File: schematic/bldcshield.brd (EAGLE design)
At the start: 51 parts, among them IC3 IR2101SMD, IC4 IR2101SMD, IC5 IR2101SMD

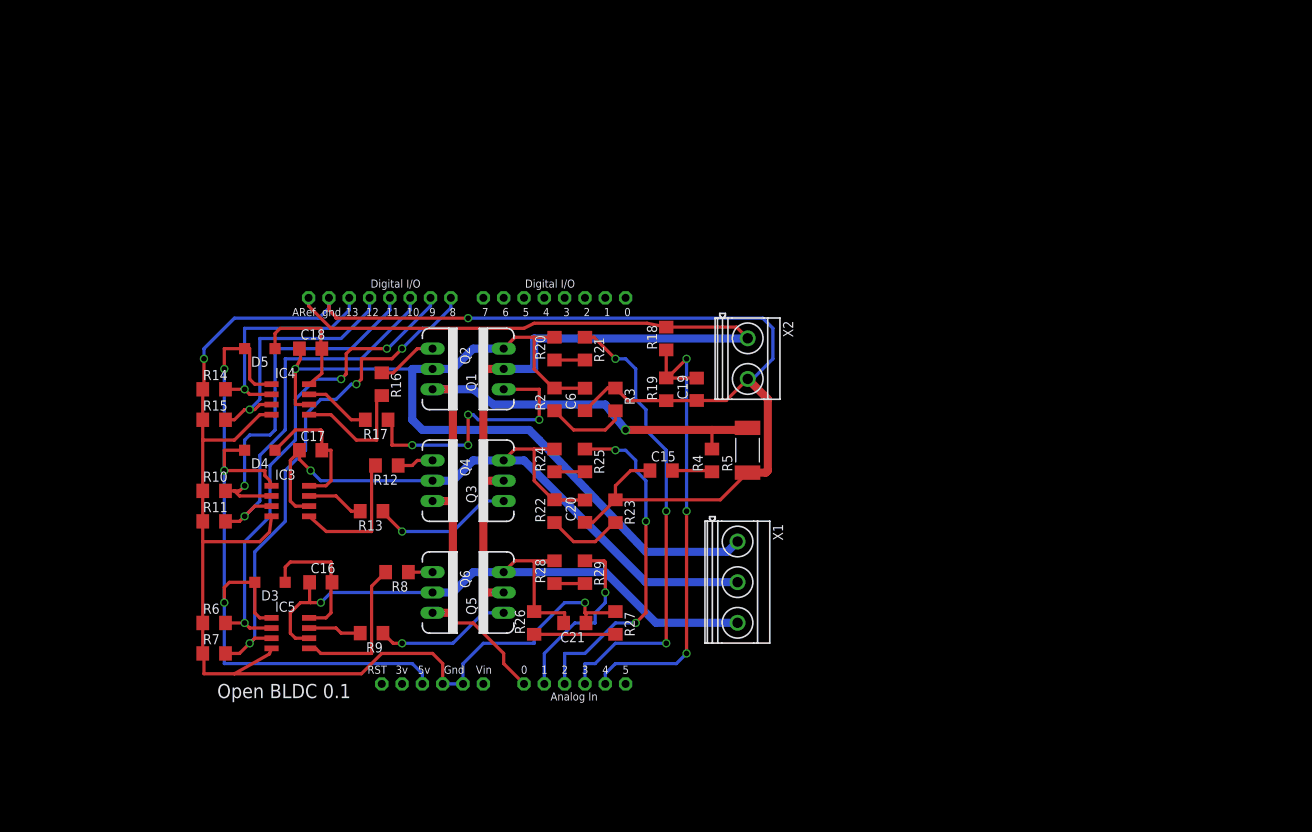
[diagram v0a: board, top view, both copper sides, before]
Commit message: redoing brf layout from scatch
deleted gerbers and backed up brd file
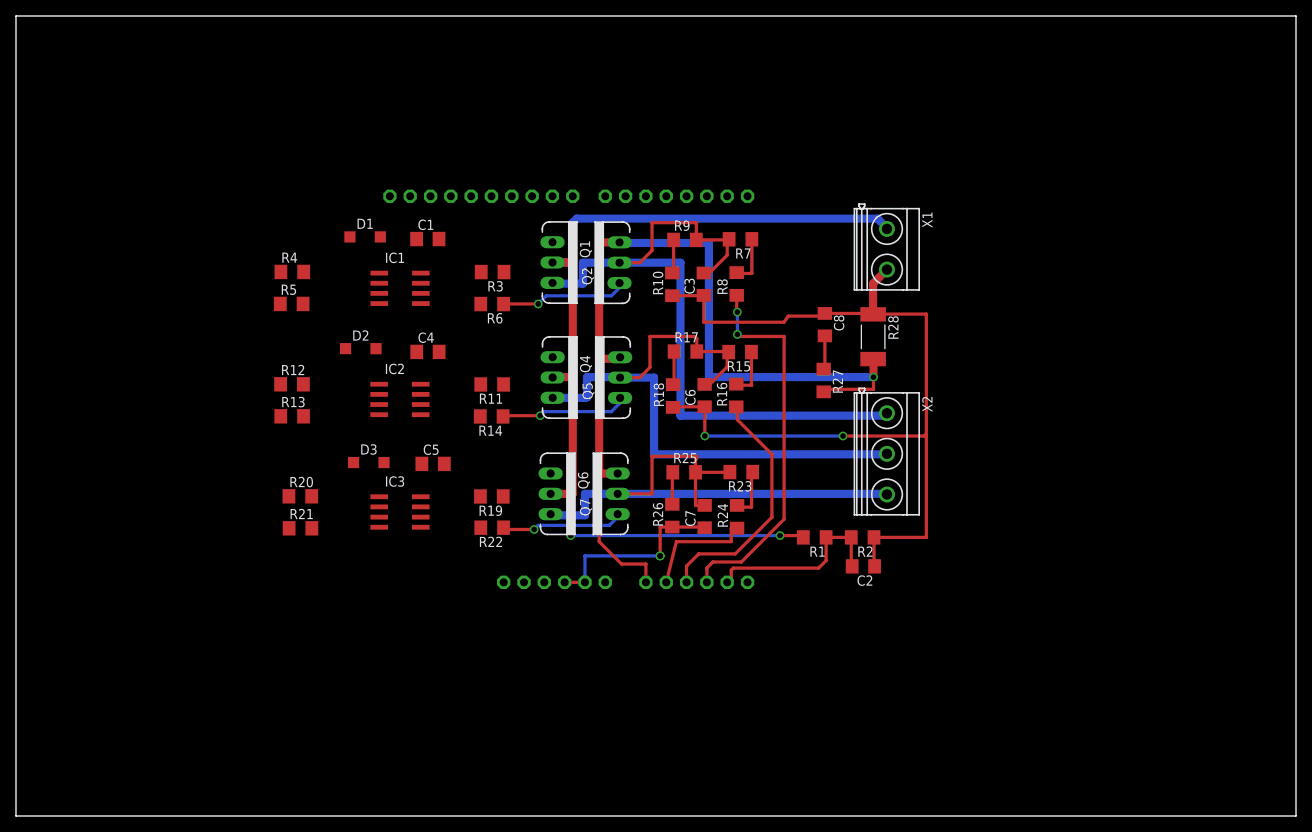
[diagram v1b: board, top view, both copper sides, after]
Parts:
- removed C15, C19: 22p, SmartPrj:C1206
- removed C16, C17, C18: 100nf, SmartPrj:C1206
- removed C20, C21: 100pF, SmartPrj:C1206
- removed D4, D5: MMSD914, diode:SOD123
- removed E$1: (no value), adafruit:ARDUINO-NOHOLE
- removed IC4, IC5: IR2101SMD, IR:SO08
- removed R29: 15k, SmartPrj:R1206
- added C1, C4, C5: 100nf, SmartPrj:C1206
- added C2, C8: 22p, SmartPrj:C1206
- added C3, C7: 100pF, SmartPrj:C1206
- added D1, D2: MMSD914, diode:SOD123
- added IC1, IC2: IR2101SMD, IR:SO08
- added Q7: (no value), SparkFun:TO220V
- added R1: 200K, SmartPrj:R1206
- Q3: value (none) -> Shield; device SparkFun:TO220V -> adafruit:ARDUINOR3-BLDC
- R10: value 10k -> 22k
- R11, R14, R6: value 10k -> 22
- R12, R13: value 22 -> 10k
- R15, R7: value 10k -> 100k
- R16, R8: value 22 -> 15k
- R17, R9: value 22 -> 22k
- R18: value 200K -> 22k
- R19: value 68k -> 22
- R2: value 22k -> 68k
- R20: value 100k -> 10k
- R21: value 15k -> 10k
- R22, R3: value 22k -> 22
- R23: value 22k -> 100k
- R24: value 100k -> 15k
- R25: value 15k -> 22k
- R27: value 22k -> 4.7k
- R28: value 100k -> 0.001; device SmartPrj:R1206 -> resistor:R2512
- R4: value 4.7k -> 10k
- R5: value 0.001 -> 10k; device resistor:R2512 -> SmartPrj:R1206
- X1: device con-phoenix-508:MKDSN1,5/3-5,08 -> con-phoenix-508:MKDSN1,5/2-5,08
- X2: device con-phoenix-508:MKDSN1,5/2-5,08 -> con-phoenix-508:MKDSN1,5/3-5,08
- moved R7 83.7 mm to (90.6, 72.1), turned to 180 degrees
- moved R15 66.3 mm to (90.5, 58.0), turned to 180 degrees
- moved R9 62.8 mm to (83.6, 72.0), turned to 0 degrees
- moved R10 62.8 mm to (82.0, 66.5), turned to 90 degrees
- moved R5 59.8 mm to (34.5, 64.0), turned to 0 degrees
- moved R4 57.5 mm to (34.5, 68.0), turned to 0 degrees
- moved R8 55.7 mm to (90.1, 66.5), turned to 90 degrees
- moved R6 52.9 mm to (59.5, 64.0), turned to 180 degrees
- moved R28 49.5 mm to (107.1, 59.9), turned to 270 degrees
- moved X1 47.9 mm to (108.8, 70.8)
- moved R16 44.3 mm to (90.0, 52.6), turned to 90 degrees
- moved R2 42.2 mm to (105.8, 34.8), turned to 180 degrees
- moved R21 42.1 mm to (35.6, 36.0), turned to 0 degrees
- moved R27 40.0 mm to (101.0, 54.4)
- moved R17 39.5 mm to (83.7, 58.1), turned to 0 degrees
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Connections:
- removed net S$2: C21.1, IC3.4, IC4.4, IC5.4, R10.1, R11.1, R14.1, R15.1, R27.1, R6.1, R7.1
- removed net S$3: C15.1, C19.1, C20.1, C6.1, R19.1, R23.1, R3.1, R5.1, X2.2
- removed net S$4: R4.2
- removed net S$5: IC3.2
- removed net S$8: E$1.D9
- new net +3V3: Q3.3V
- new net GND: C2.1, C3.1, C6.1, C7.1, C8.1, IC1.4, IC2.4, IC3.4, Q3.GND, Q3.GND1, Q3.GND2, R10.1, R12.1, R13.1, R18.1, R2.1, R20.1, R21.1, R26.1, R28.1, R4.1, R5.1, X1.2
- net +5V: now also D1.A, D2.A, IC1.1, IC2.1, Q3.5V, Q3.VIN; no longer D4.A, D5.A, IC4.1, IC5.1
- net BLDC1: now also C1.1, C3.2, IC1.6, R7.2, R9.2, X2.1; no longer C18.1, C6.2, IC4.6, R2.2, R20.2, X1.1
- net BLDC2: now also C4.1, C6.2, IC2.6, Q4.3, Q5.2, R15.2, R17.2, X2.2; no longer C17.1, C20.2, IC3.6, Q3.3, Q4.2, R22.2, R24.2, X1.2
- net BLDC3: now also C5.1, C7.2, IC3.6, Q6.3, Q7.2, R23.2, R25.2, X2.3; no longer C16.1, C21.2, IC5.6, Q5.3, Q6.2, R26.2, R28.2, X1.3
- net CURRENT: now also Q3.A0, Q5.3, Q7.3, R27.2, R28.2; no longer Q4.3, Q6.3
- net EMF1: now also Q3.A3, R8.1; no longer R21.1
- net EMF2: now also Q3.A2, R16.1; no longer R25.1
- net EMF3: now also Q3.A1, R24.1; no longer R29.1
- net HI_1: now also IC1.3, Q3.D12, R5.2; no longer E$1.D12, IC4.3, R15.2
- net HI_2: now also IC2.3, Q3.D10, R13.2; no longer IC3.3, R11.2
- net HI_3: now also IC3.3, Q3.D8, R21.2; no longer E$1.D8, IC5.3, R7.2
- net LOW_VOLTAGE: now also C2.2, Q3.A4, R1.1, R2.2; no longer C19.2, R18.1, R19.2
- net LO_1: now also IC1.2, Q3.D13, R4.2; no longer E$1.D13, IC4.2, R14.2
- net LO_2: now also IC2.2, Q3.D11, R12.2; no longer E$1.D11
- net LO_3: now also IC3.2, Q3.D9, R20.2; no longer IC5.2, R6.2
- net N$1: now also Q4.1, R11.1; no longer Q3.1, R13.1
- net N$10: now also R7.1, R8.2; no longer R20.1, R21.2
- net N$12: now also R17.1, R18.2; no longer R22.1, R23.2
- net N$13: now also IC3.7, R19.2; no longer IC5.7, R9.2
- net N$14: now also Q6.1, R19.1; no longer Q5.1, R9.1
- net N$15: now also Q7.1, R22.1; no longer Q6.1, R8.1
- net N$16: now also IC3.5, R22.2; no longer IC5.5, R8.2
- net N$17: now also C5.2, IC3.8; no longer C16.2, IC5.8
- net N$19: now also R15.1, R16.2; no longer R24.1, R25.2
- net N$2: now also R10.2, R9.1; no longer R2.1, R3.2
- net N$21: now also IC2.7, R11.2; no longer IC3.7, R13.2
- net N$23: now also Q5.1, R14.1; no longer Q4.1, R12.1
- net N$24: now also IC2.5, R14.2; no longer IC3.5, R12.2
- net N$25: now also C4.2, D2.C, IC2.8; no longer C17.2, D4.C, IC3.8
- net N$26: now also R25.1, R26.2; no longer R26.1, R27.2
- net N$28: now also R23.1, R24.2; no longer R28.1, R29.2
- net N$29: now also IC1.7, R3.2; no longer IC4.7, R17.2
- net N$30: now also R3.1; no longer R17.1
- net N$31: now also R6.1; no longer R16.1
- net N$32: now also IC1.5, R6.2; no longer IC4.5, R16.2
- net N$33: now also C1.2, D1.C, IC1.8; no longer C18.2, D5.C, IC4.8
- net N$9: now also C8.2, R27.1; no longer C15.2, R4.1
- net VCC: now also Q3.AREF, Q4.2, Q6.2, R1.2, X1.1; no longer Q3.2, Q5.2, R18.2, X2.1
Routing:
- net S$2: track 150.9 -> 0.00 mm, vias 1 -> 0
- net GND: track 0.00 -> 141.0 mm, vias 0 -> 3
- net S$3: track 127.4 -> 0.00 mm, vias 1 -> 0
- net +5V: track 100.4 -> 0.00 mm, vias 3 -> 0
- net HI_3: track 64.5 -> 0.00 mm, vias 3 -> 0
- net LO_3: track 52.1 -> 0.00 mm, vias 3 -> 0
- net HI_2: track 48.0 -> 0.00 mm
- net LO_2: track 45.0 -> 0.00 mm, vias 1 -> 0
- net LOW_VOLTAGE: track 60.2 -> 23.8 mm, vias 3 -> 0
- net N$30: track 34.1 -> 0.00 mm, vias 4 -> 0
- net HI_1: track 31.4 -> 0.00 mm, vias 1 -> 0
- net LO_1: track 28.7 -> 0.00 mm, vias 1 -> 0
- net CURRENT: track 92.4 -> 113.2 mm
- net N$16: track 19.0 -> 0.00 mm
- net BLDC1: track 108.9 -> 90.5 mm, vias 1 -> 0
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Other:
- board outline added: 160 x 100 mm
- board text removed: "Open BLDC 0.1"
- board text removed: "www.OpenRover.com"
